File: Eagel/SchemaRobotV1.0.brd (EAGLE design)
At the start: 160 x 100 mm, 25 parts

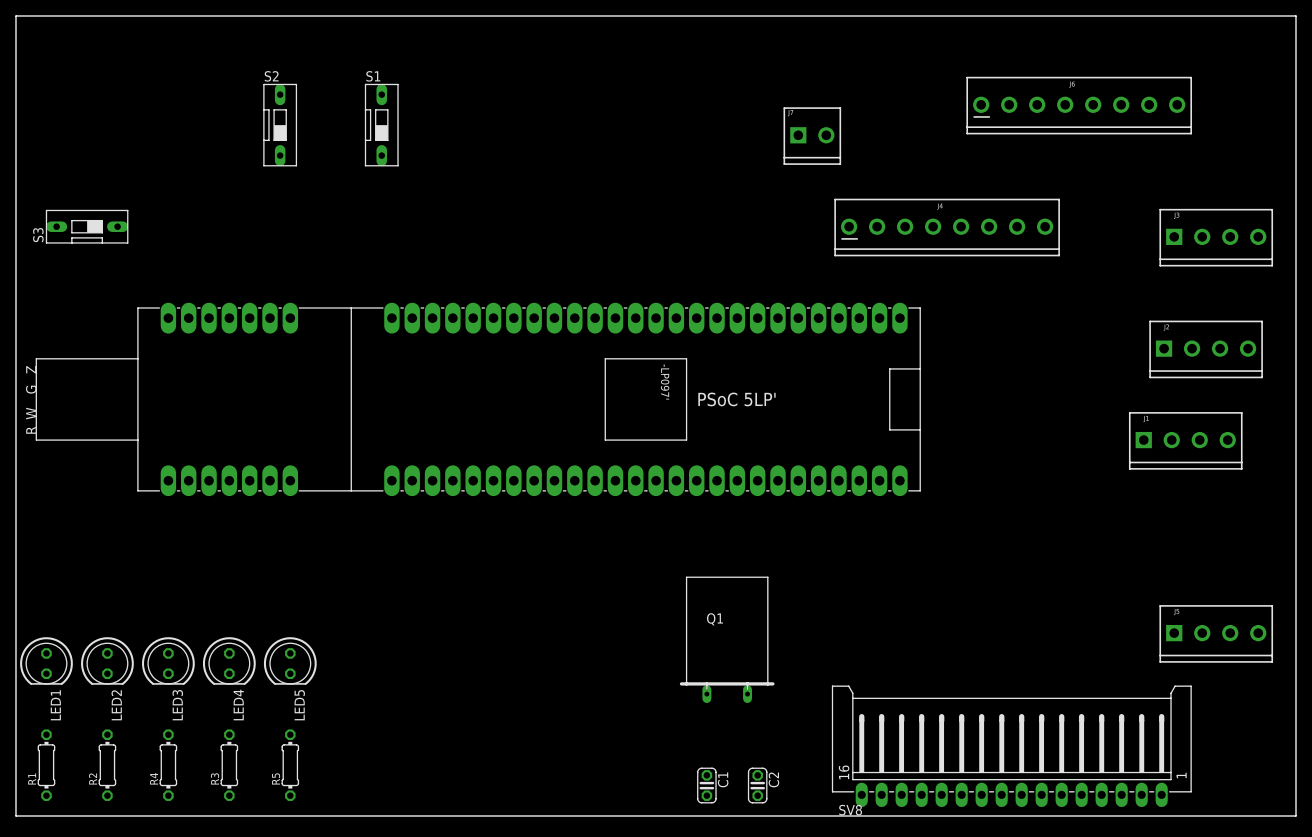
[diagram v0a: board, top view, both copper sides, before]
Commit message: eagle
schema bijna af!
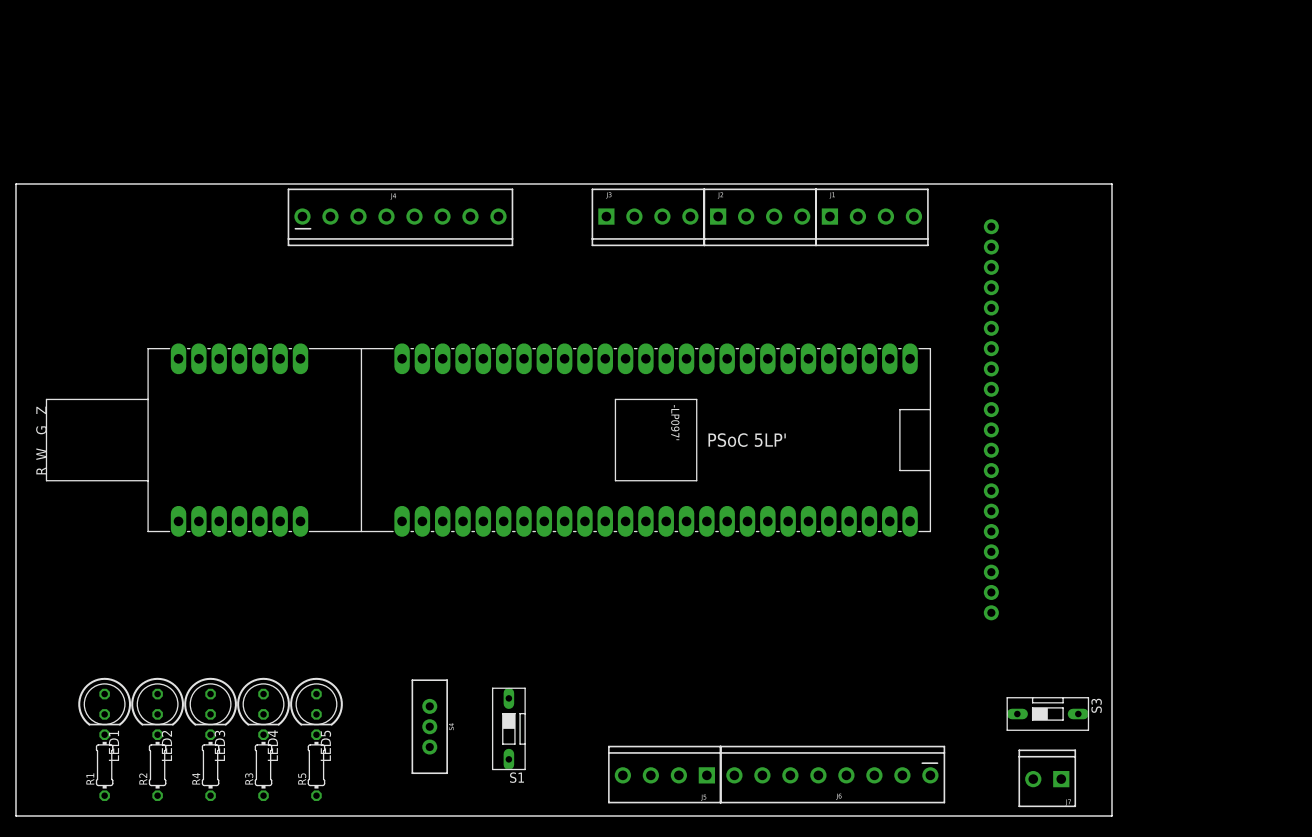
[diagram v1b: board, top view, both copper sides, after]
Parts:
- removed C1, C2: (no value), rcl:C025-024X044
- removed Q1: (no value), special:Q
- removed S2: (no value), switch-dil:DS-01
- removed SV8: (no value), con-amp-mt:L16P
- added J8: Connector LCD, SparkFun-Connectors:1X20
- added S4: (no value), SparkFun-Switches:SWITCH_SPDT_PTH_11.6X4.0MM
- J1: value (none) -> Connector US1
- J2, J3: value (none) -> Connector US 2
- J4: value (none) -> Connector H-Brug
- J5: value (none) -> Connector IR voeding
- J6: value (none) -> Connector IR signalen
- J7: value (none) -> Connector batterij 12v
- R1, R2, R3, R4, R5: value (none) -> 100 ohm
- moved S3 134.7 mm to (129.0, 12.8), turned to 270 degrees
- moved J7 86.9 mm to (130.7, 4.61), turned to 180 degrees
- moved J6 84.1 mm to (114.3, 5.08), turned to 180 degrees
- moved S1 77.1 mm to (61.6, 10.9), turned to 180 degrees
- moved J3 71.0 mm to (73.8, 74.9)
- moved J4 68.3 mm to (35.8, 74.9)
- moved J5 61.1 mm to (86.4, 5.08), turned to 180 degrees
- moved J2 58.1 mm to (87.8, 74.9)
- moved J1 48.2 mm to (101.7, 74.9)
- moved LED1 8.87 mm to (11.1, 14.0)
- moved LED2 8.07 mm to (17.7, 14.0)
- moved LED3 7.32 mm to (24.3, 14.0)
- moved R1 7.27 mm to (11.1, 6.35)
- moved LED4 6.64 mm to (30.9, 14.0)
- moved R2 6.27 mm to (17.7, 6.35)
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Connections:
- removed net ECHO: DEVICE1.P1.0/SWDIO, DEVICE1.P12.1/I2C(SDA), DEVICE1.P12.3, J1.3, J2.3, J3.3
- removed net IRS: DEVICE1.P2.3, J6.6
- removed net N$15: DEVICE1.P0.1, SV8.13
- removed net N$16: DEVICE1.P0.0, SV8.14
- removed net N$17: C1.1, DEVICE1.P15.2/XTAL_OUT, Q1.1
- removed net N$18: C2.1, DEVICE1.P15.3/XTAL_IN, Q1.2
- removed net N$21: J6.4
- removed net TRIG: DEVICE1.P1.1/SWDCLK, DEVICE1.P12.0/I2C(SCL), DEVICE1.P12.2, J1.2, J2.2, J3.2
- new net ECHO1: DEVICE1.P12.3, J1.3
- new net ECHO2: DEVICE1.P12.1/I2C(SDA), J2.3
- new net ECHO3: DEVICE1.P1.0/SWDIO, J3.3
- new net IRS3: DEVICE1.P0.5, J6.3
- new net IRS5: DEVICE1.P0.3/EXT_REF0, J6.5
- new net N$1: DEVICE1.P2.3, J8.14
- new net N$7: DEVICE1.P2.2/SW1, J8.13
- new net TRIG1: DEVICE1.P12.2, J1.2
- new net TRIG2: DEVICE1.P12.0/I2C(SCL), J2.2
- new net TRIG3: DEVICE1.P1.1/SWDCLK, J3.2
- net GND: now also J5.3, J5.4, J8.1, J8.3, S4.3; no longer C1.2, C2.2, J5.1, SV8.1, SV8.3
- net IRS1: now also DEVICE1.P0.7, J6.1; no longer DEVICE1.P2.1/LED1, J6.8
- net IRS2: now also DEVICE1.P0.6, J6.2; no longer DEVICE1.P2.2/SW1, J6.7
- net IRS4: now also DEVICE1.P0.4/SAR0, J6.4; no longer J6.5
- net IRS6: now also DEVICE1.P0.2/SAR1, J6.6; no longer DEVICE1.P2.6, J6.3
- net IRS7: now also DEVICE1.P0.1, J6.7; no longer DEVICE1.P2.7, J6.2
- net IRS8: now also DEVICE1.P0.0, J6.8; no longer J6.1
- net LEDON: now also DEVICE1.P3.7; no longer DEVICE1.P2.0
- net N$10: now also DEVICE1.P2.4, J8.6; no longer DEVICE1.P0.4/SAR0, SV8.6
- net N$11: now also DEVICE1.P2.6, J8.5; no longer DEVICE1.P0.3/EXT_REF0, SV8.11
- net N$12: now also DEVICE1.P2.5, J8.4; no longer DEVICE1.P0.2/SAR1, SV8.12
- net N$8: now also DEVICE1.P2.1/LED1, J8.12; no longer DEVICE1.P0.6, SV8.4
- net N$9: now also DEVICE1.P2.0, J8.11; no longer DEVICE1.P0.5, SV8.5
- net SW1: now also S4.2; no longer S2.1
- net VCC: now also J5.1, J8.2, S4.1; no longer J5.3, S2.2, SV8.2
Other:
- board size 160 x 100 mm -> 137 x 79 mm
